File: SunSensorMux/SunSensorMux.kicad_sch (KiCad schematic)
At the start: 7 parts, among them U1 TCA9548A_Multiplexer, U2 FEATHER_M0_BASIC_PROTO

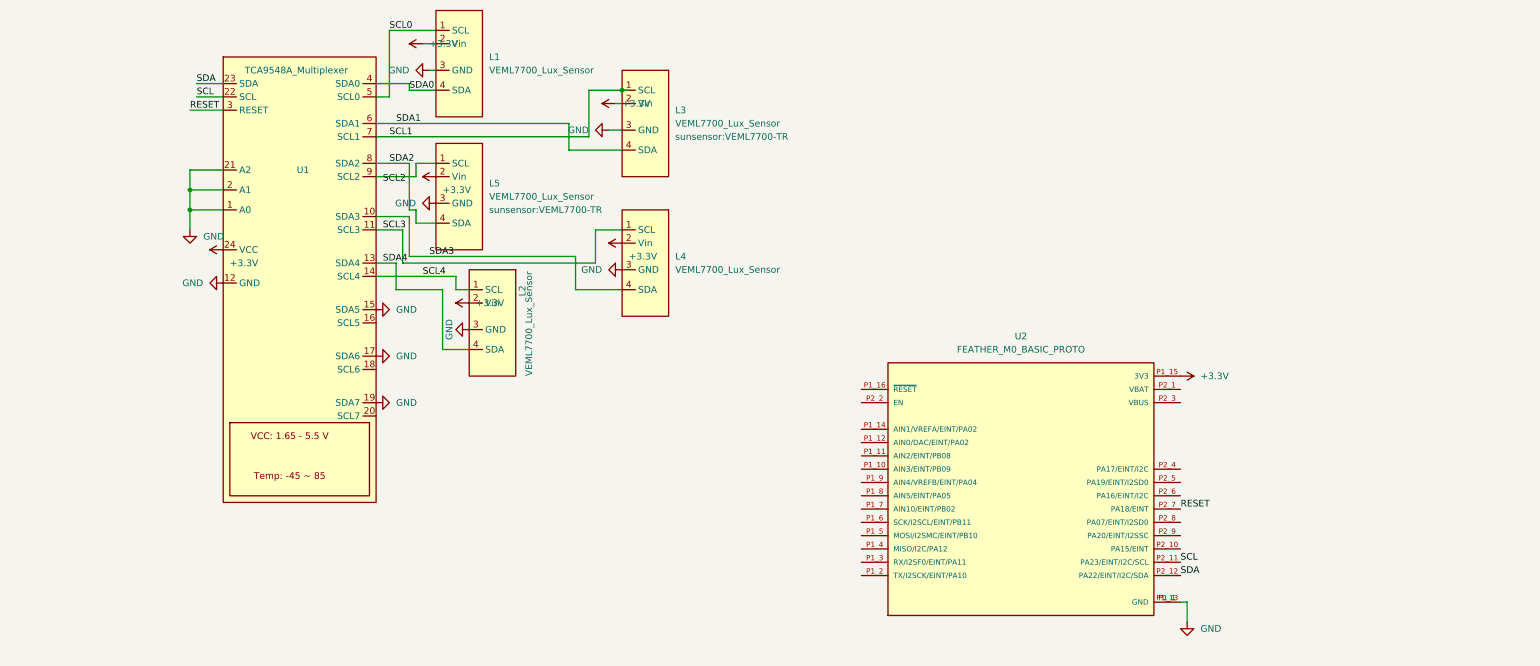
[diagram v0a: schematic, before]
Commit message: Finish Routing
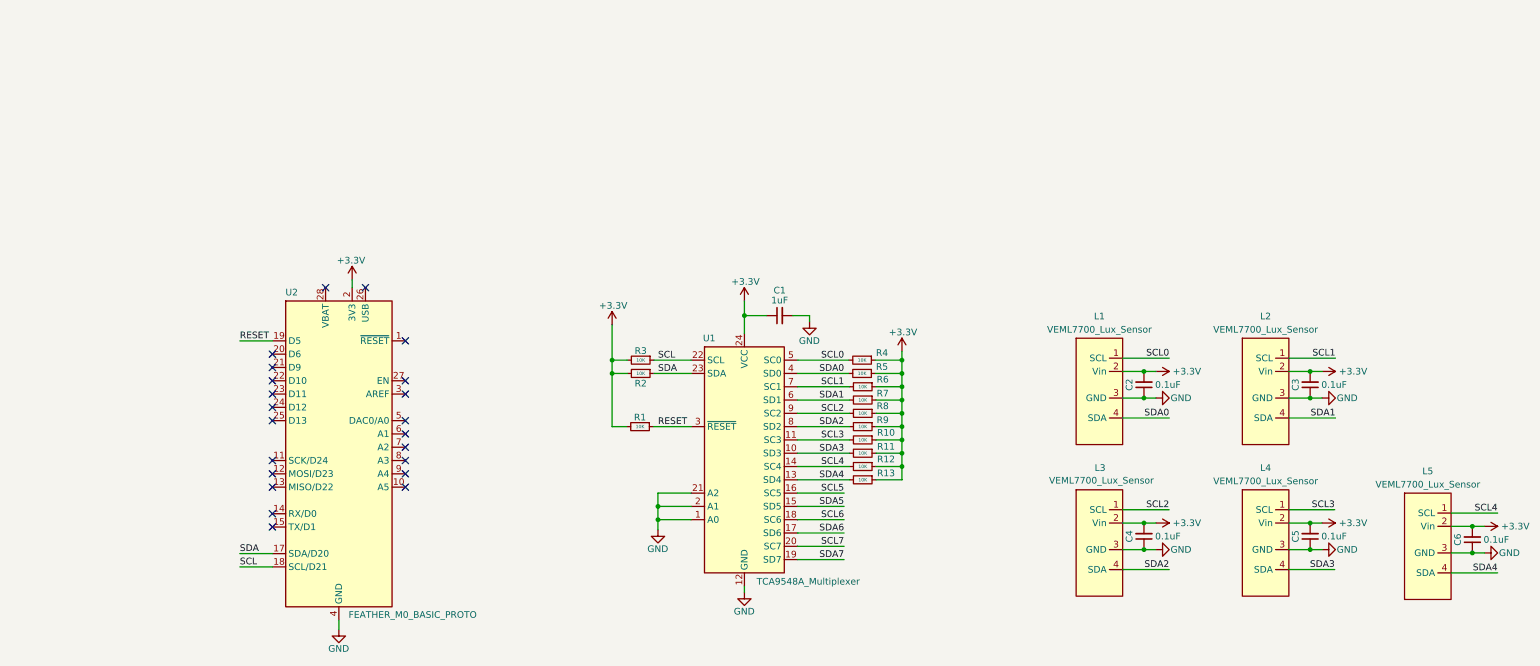
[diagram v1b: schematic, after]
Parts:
- removed L2, L4, L5: VEML7700_Lux_Sensor, sunsensor:VEML7700-TR, symbol Sensor_Optical:VEML7700_Lux_Sensor
- added C1: 1uF, Capacitor_SMD:C_0603_1608Metric, symbol Device:C_Small
- added C2, C3, C4, C5, C6: 0.1uF, Capacitor_SMD:C_0603_1608Metric, symbol Device:C_Small
- added L2, L4, L5: VEML7700_Lux_Sensor, sunsensor:VEML7700-TT, symbol SunSensor:VEML7700_Lux_Sensor
- added R1, R10, R11, R12, R13, R2, R3, R4, R5, R6, R7, R8, R9: 10K, Resistor_SMD:R_0603_1608Metric, symbol Device:R_Small
- L1, L3: footprint sunsensor:VEML7700-TR -> sunsensor:VEML7700-TT; symbol Sensor_Optical:VEML7700_Lux_Sensor -> SunSensor:VEML7700_Lux_Sensor
- U1: footprint sunsensor:SOP65P640X120-24N -> Package_SO:TSSOP-24_4.4x7.8mm_P0.65mm; symbol Analog_Switch:TCA9548A_Multiplexer -> Interface_Expansion:TCA9548APWR
- U2: footprint sunsensor:MODULE_FEATHER_M0_BASIC_PROTO -> Module:Adafruit_Feather; symbol sunsensor:FEATHER_M0_BASIC_PROTO -> MCU_Module:Adafruit_Feather_M0_Basic_Proto
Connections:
- net GND: now also U2.16 (GND), U2.4 (GND), C1.2, C2.1, C3.1, C4.1, C5.1, C6.1, L2.3 (GND), L4.3 (GND), L5.3 (GND); no longer U1.15 (SDA5), U1.17 (SDA6), U1.19 (SDA7), U2.P1_1 (GND), U2.P1_13 (GND)
- net RESET: now also U2.19 (D5), R1.1; no longer U2.P2_7 (PA18/EINT)
- net SCL: now also U2.18 (SCL/D21), R3.1; no longer U2.P2_11 (PA23/EINT/I2C/SCL)
- net SCL0: now also R4.2
- net SCL1: now also L2.1 (SCL), R6.2; no longer L3.1 (SCL)
- net SCL2: now also L3.1 (SCL), U1.9 (SC2), R8.2
- net SCL3: now also L4.1 (SCL), R10.2
- net SCL4: now also L5.1 (SCL), R12.2
- net SDA: now also U2.17 (SDA/D20), R2.1; no longer U2.P2_12 (PA22/EINT/I2C/SDA)
- net SDA0: now also R5.2
- net SDA1: now also L2.4 (SDA), R7.2; no longer L3.4 (SDA)
- net SDA2: now also L3.4 (SDA), R9.2
- net SDA3: now also L4.4 (SDA), R11.2
- net SDA4: now also L5.4 (SDA), R13.2
- net SCL5: now reaches U1.16 (SC5)
- net SCL6: now reaches U1.18 (SC6)
- net SCL7: now reaches U1.20 (SC7)
- net +3V3 renamed +3.3V
- net +3.3V: now also U2.2 (3V3), C1.1, C2.2, C3.2, C4.2, C5.2, C6.2, L2.2 (Vin), L4.2 (Vin), L5.2 (Vin), R1.2, R10.1, R11.1, R12.1, R13.1, R2.2, R3.2, R4.1, R5.1, R6.1, R7.1, R8.1, R9.1; no longer U2.P1_15 (3V3)
- new net SDA5: U1.15 (SD5)
- new net SDA6: U1.17 (SD6)
- new net SDA7: U1.19 (SD7)
- no-connect marks 0 -> 22
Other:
- moved on the sheet: L1, L3
